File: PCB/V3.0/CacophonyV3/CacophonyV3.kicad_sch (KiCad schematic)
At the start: 25 parts, among them J1 Conn_01x04, J2 Conn_01x05, J3 Conn_01x03, J4 Conn_01x03, J5 Conn_01x03, J6 Conn_01x02

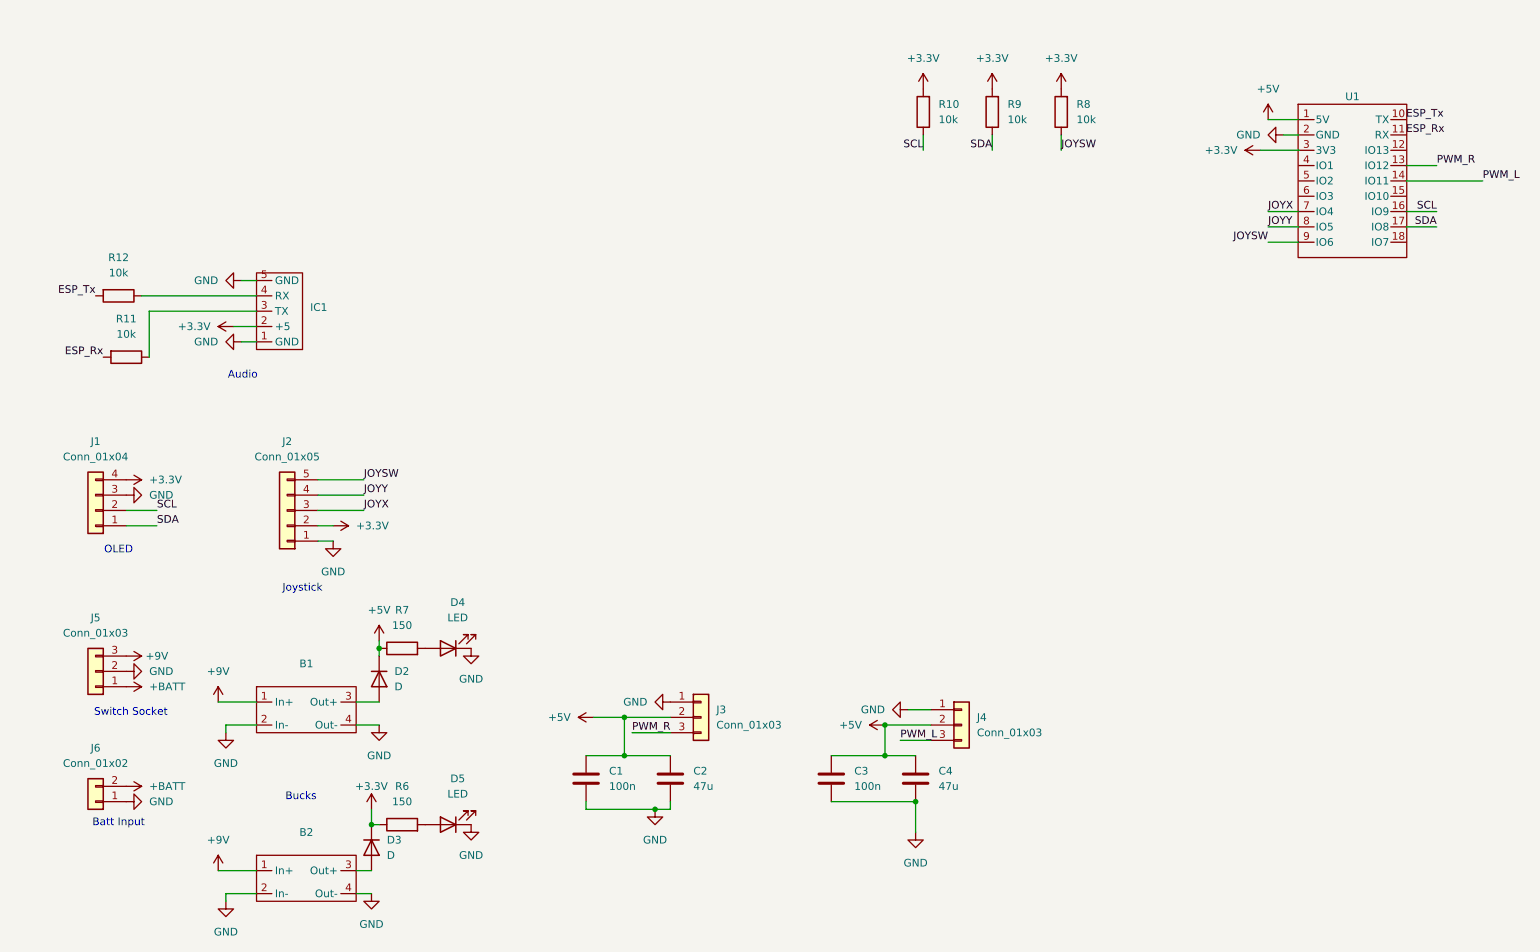
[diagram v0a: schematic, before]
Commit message: New PCB
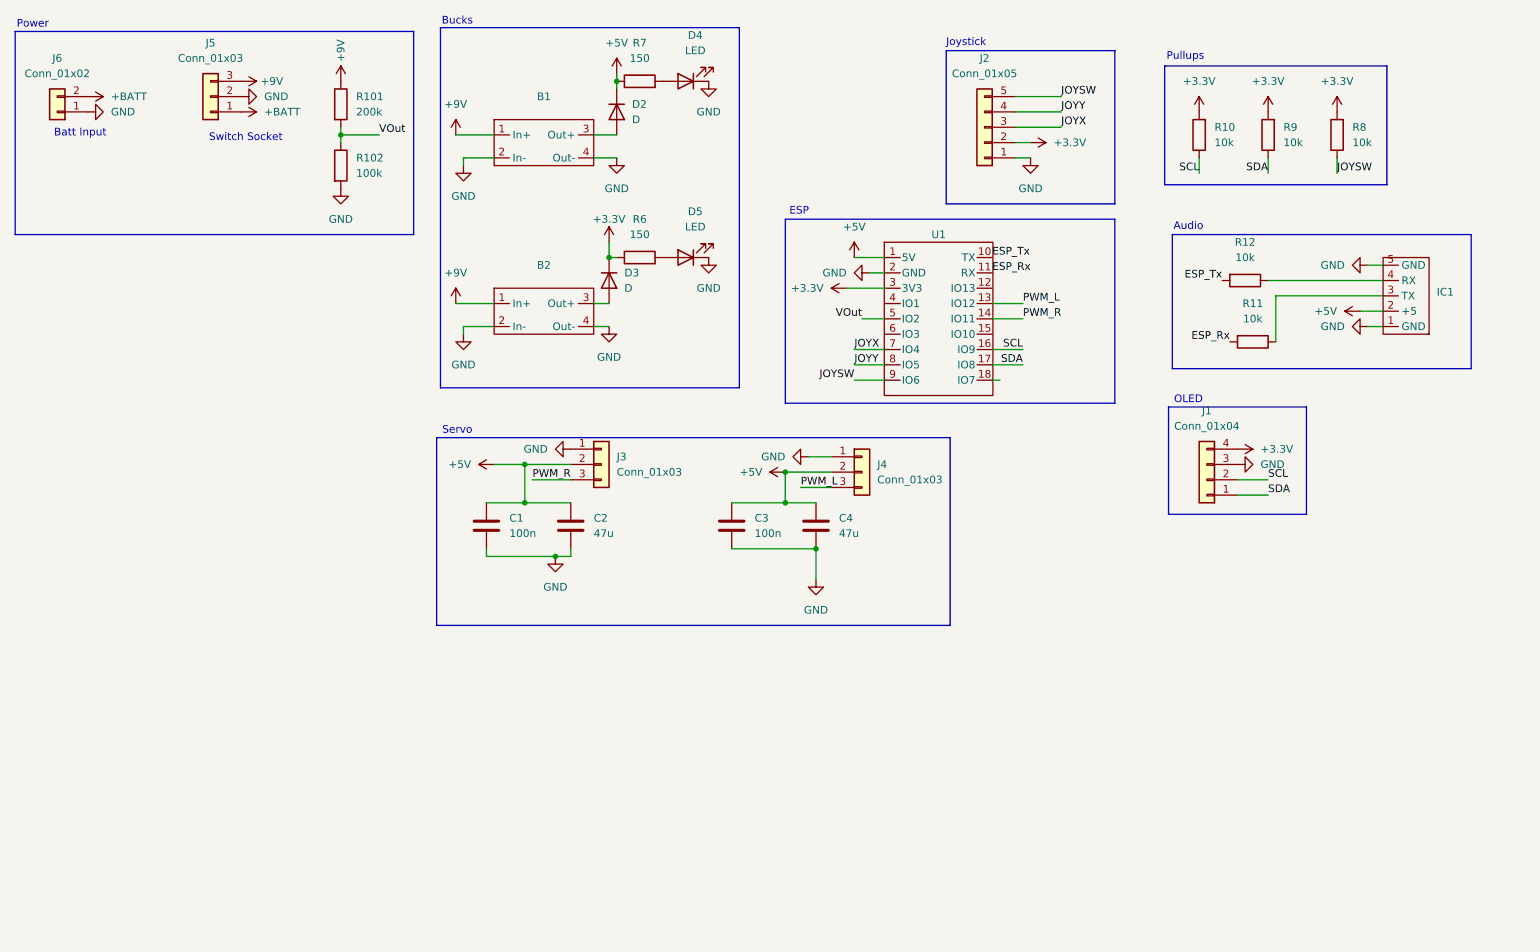
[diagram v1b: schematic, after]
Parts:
- added R101: 200k, Resistor_SMD:R_0402_1005Metric, symbol Device:R
- added R102: 100k, Resistor_SMD:R_0402_1005Metric, symbol Device:R
- C1, C2, C3, C4: footprint Capacitor_SMD:C_1206_3216Metric -> Resistor_SMD:R_0402_1005Metric
- D4, D5: footprint LED_SMD:LED_0603_1608Metric -> LED_SMD:LED_0402_1005Metric
- R10, R11, R12, R6, R8, R9: footprint Resistor_SMD:R_2512_6332Metric -> Resistor_SMD:R_0402_1005Metric
- R7: footprint Resistor_SMD:R_2512_6332Metric -> Capacitor_SMD:C_0402_1005Metric
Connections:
- net +3.3V: no longer IC1.2 (+5)
- net +5V: now also IC1.2 (+5)
- net +9V: now also R101.1
- net GND: now also R102.2
- net PWM_L: now also U1.13 (IO12); no longer U1.14 (IO11)
- net PWM_R: now also U1.14 (IO11); no longer U1.13 (IO12)
- net VOut: now reaches U1.5 (IO2)
- net VOut: now also R101.2, R102.1
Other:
- note added: "ESP"
- note added: "Power"
- note added: "Pullups"
- note added: "Servo"
- moved on the sheet: B1, B2, C1, C2, C3, C4, D2, D3, D4, D5, IC1, J1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
